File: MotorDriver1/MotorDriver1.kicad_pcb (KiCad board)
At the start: 2 copper layers, 60.5 x 66.5 mm, 74 parts, among them IC1 STM32C092RCT6, IC2 mcp6004-e_p, J1 GT-USB-7010ASV, J2 Conn_01x02, J3 Conn_01x02, Q1 IRLZ44N, Q2 IRLZ44N, Q3 IRLZ44N, Q4 IRLZ44N, SW1 K2-6639SP-C4SC-04, SW2 K2-6639SP-C4SC-04, SW3 K2-6639SP-C4SC-04, U1 TPS22916CNYFPR, U2 CH340X, U3 XIAO-ESP32-C5-DIP, U4 MCP2562FDT-H/SN, U5 MCP2562FDT-H/SN, Y1 48 MHz, Y2 32.768 kHz

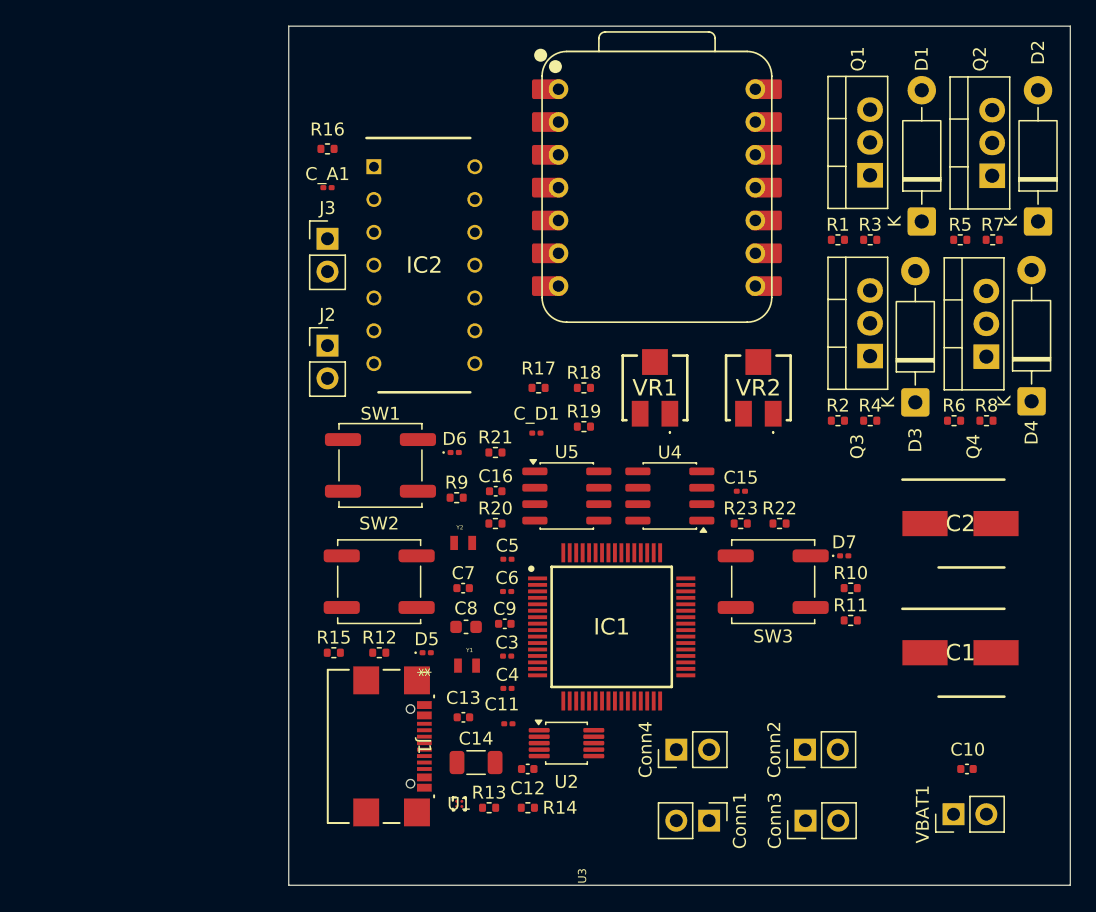
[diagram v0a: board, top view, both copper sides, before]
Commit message: Re-layed out eo stuff
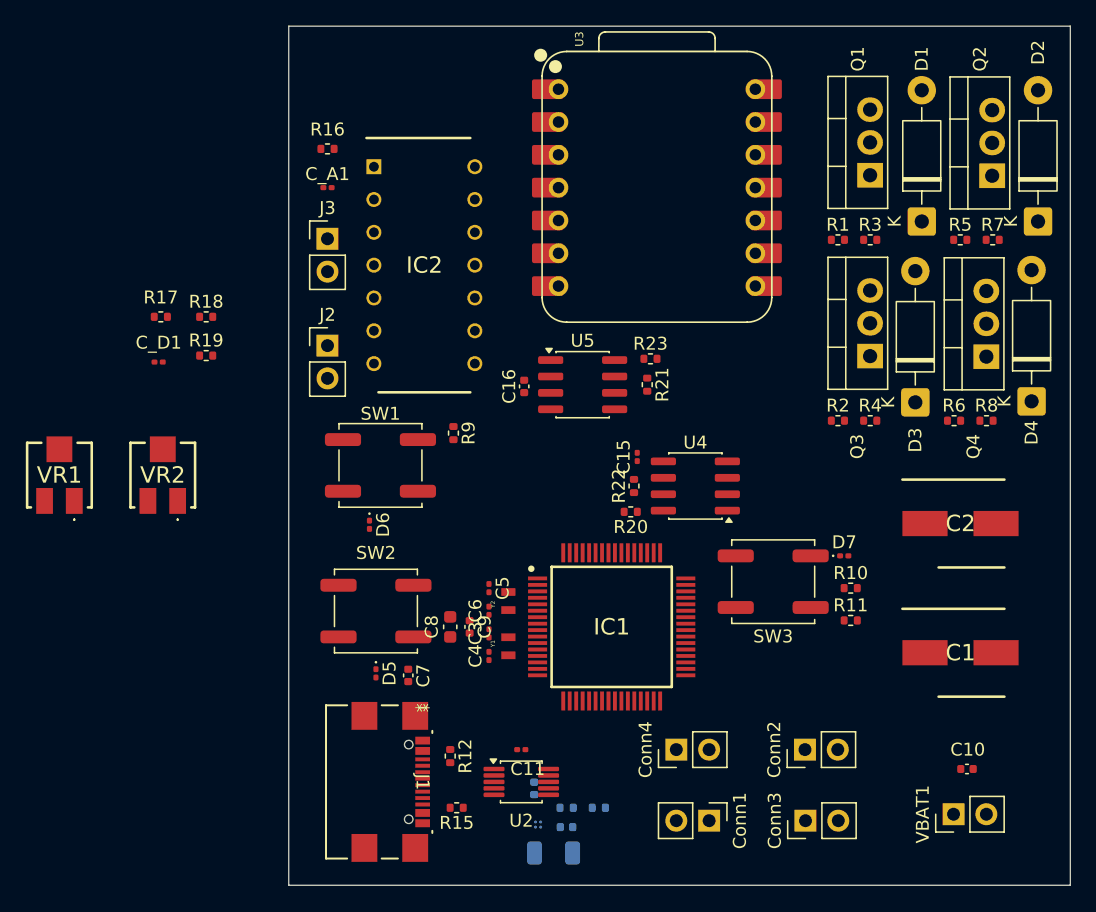
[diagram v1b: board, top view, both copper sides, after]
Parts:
- C12, C13, C14, R13, R14, U1: moved to B.Cu
- moved VR1 46.6 mm to (129.2, 60.8)
- moved VR2 46.6 mm to (137.2, 60.8)
- moved R17 29.8 mm to (137.1, 48.5)
- moved C_D1 29.8 mm to (136.9, 52.0)
- moved R18 29.8 mm to (140.6, 48.5)
- moved R19 29.8 mm to (140.6, 51.5)
- moved R15 15.3 mm to (160.0, 86.5), turned to 180 degrees
- moved R23 14.5 mm to (175.0, 51.8)
- moved R21 12.9 mm to (174.8, 53.8), turned to -90 degrees
- moved C13 11.7 mm to (168.5, 88.0)
- moved R22 11.6 mm to (173.7, 61.6), turned to 90 degrees
- moved R20 10.5 mm to (173.5, 63.6), turned to 180 degrees
- moved R12 9.70 mm to (159.5, 82.5), turned to -90 degrees
- moved C14 9.22 mm to (167.5, 90.0)
- moved U5 8.70 mm to (169.8, 53.8)
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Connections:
- IC1 pad 1: unconnected-(IC1-PC11-Pad1) -> USER_BTN
- IC1 pad 3: USER_BTN -> unconnected-(IC1-PC13-Pad3)
- U4 pad 4: FDCAN_STM -> FDCAN_RX_STM
